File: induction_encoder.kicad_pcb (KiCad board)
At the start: 4 copper layers, 136 x 136 mm, 72 parts, among them J2 Conn_01x06, U1 MT9105ET, U10 IPS2200, U11 ADS1115IDGS, U12 ADS1115IDGS, U2 MT9105ET, U3 MT9105ET, U4 MT9105ET, U5 MT9105ET, U6 MT9105ET, U7 ADS1115IDGS, U8 MT9105ET, U9 MT9105ET

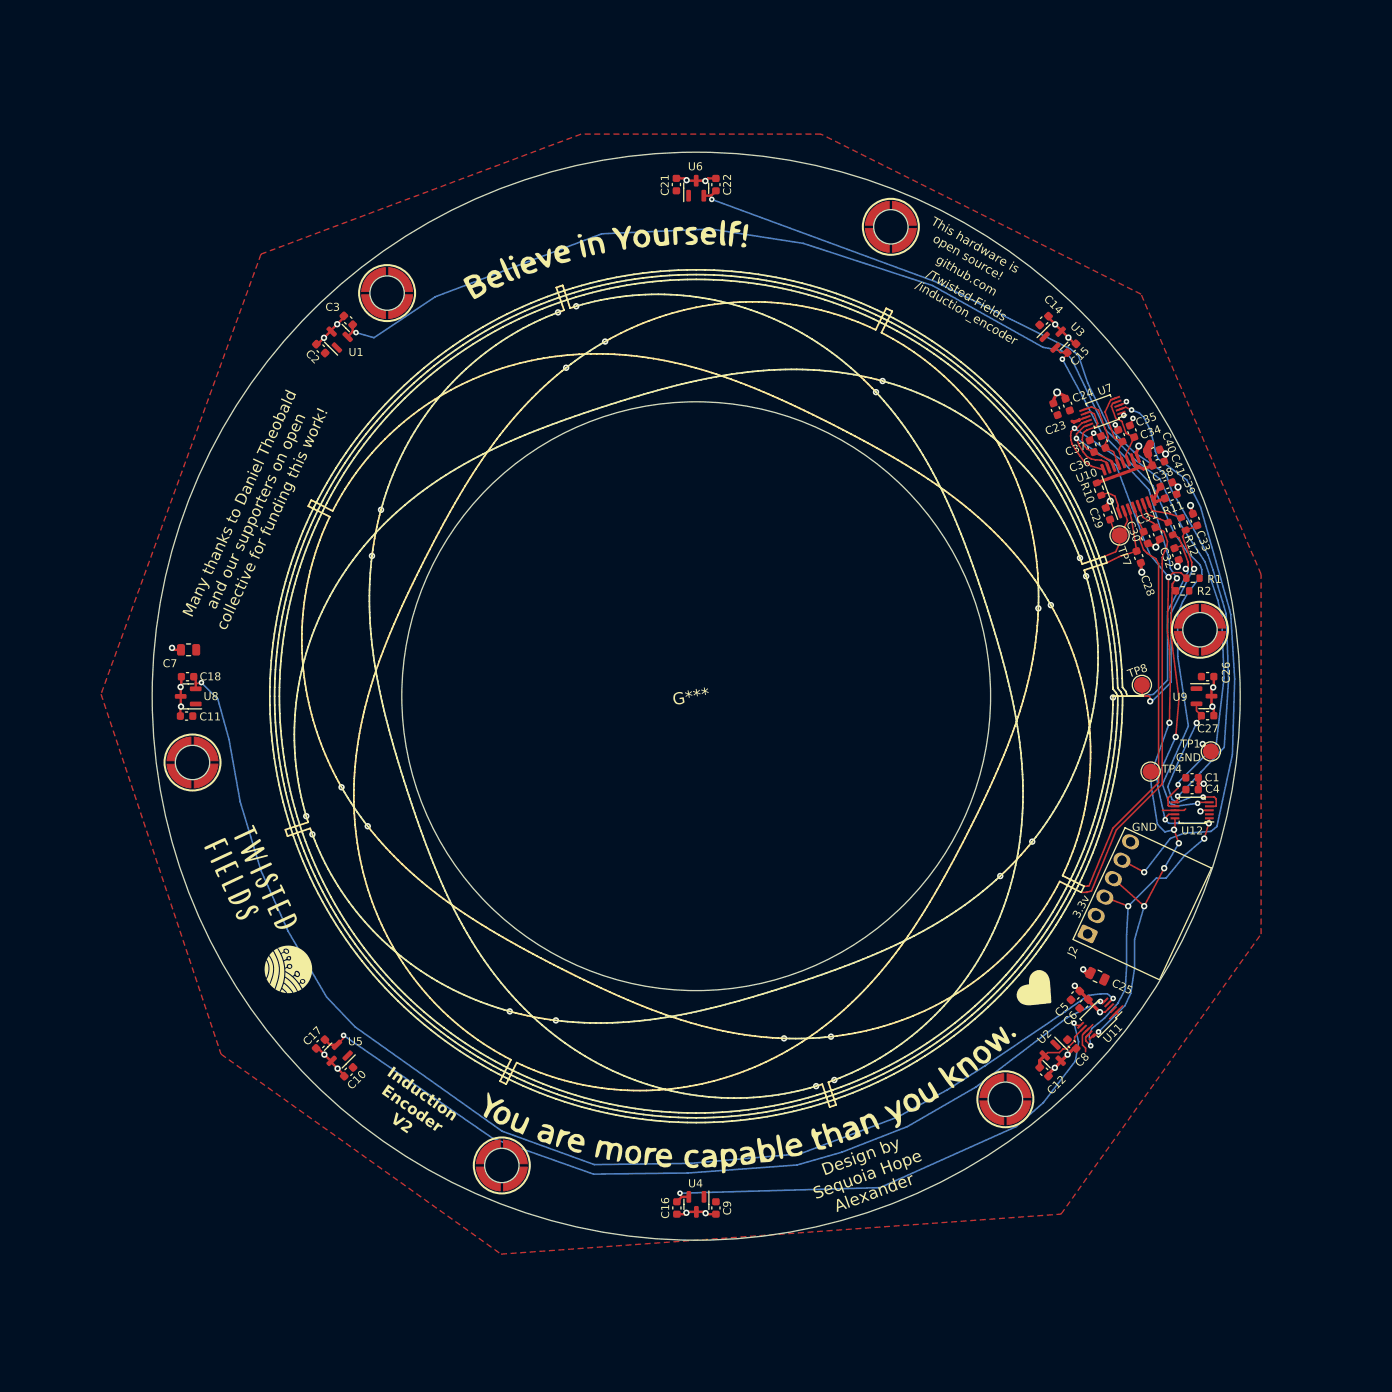
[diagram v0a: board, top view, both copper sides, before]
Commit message: changes for the 170mm design
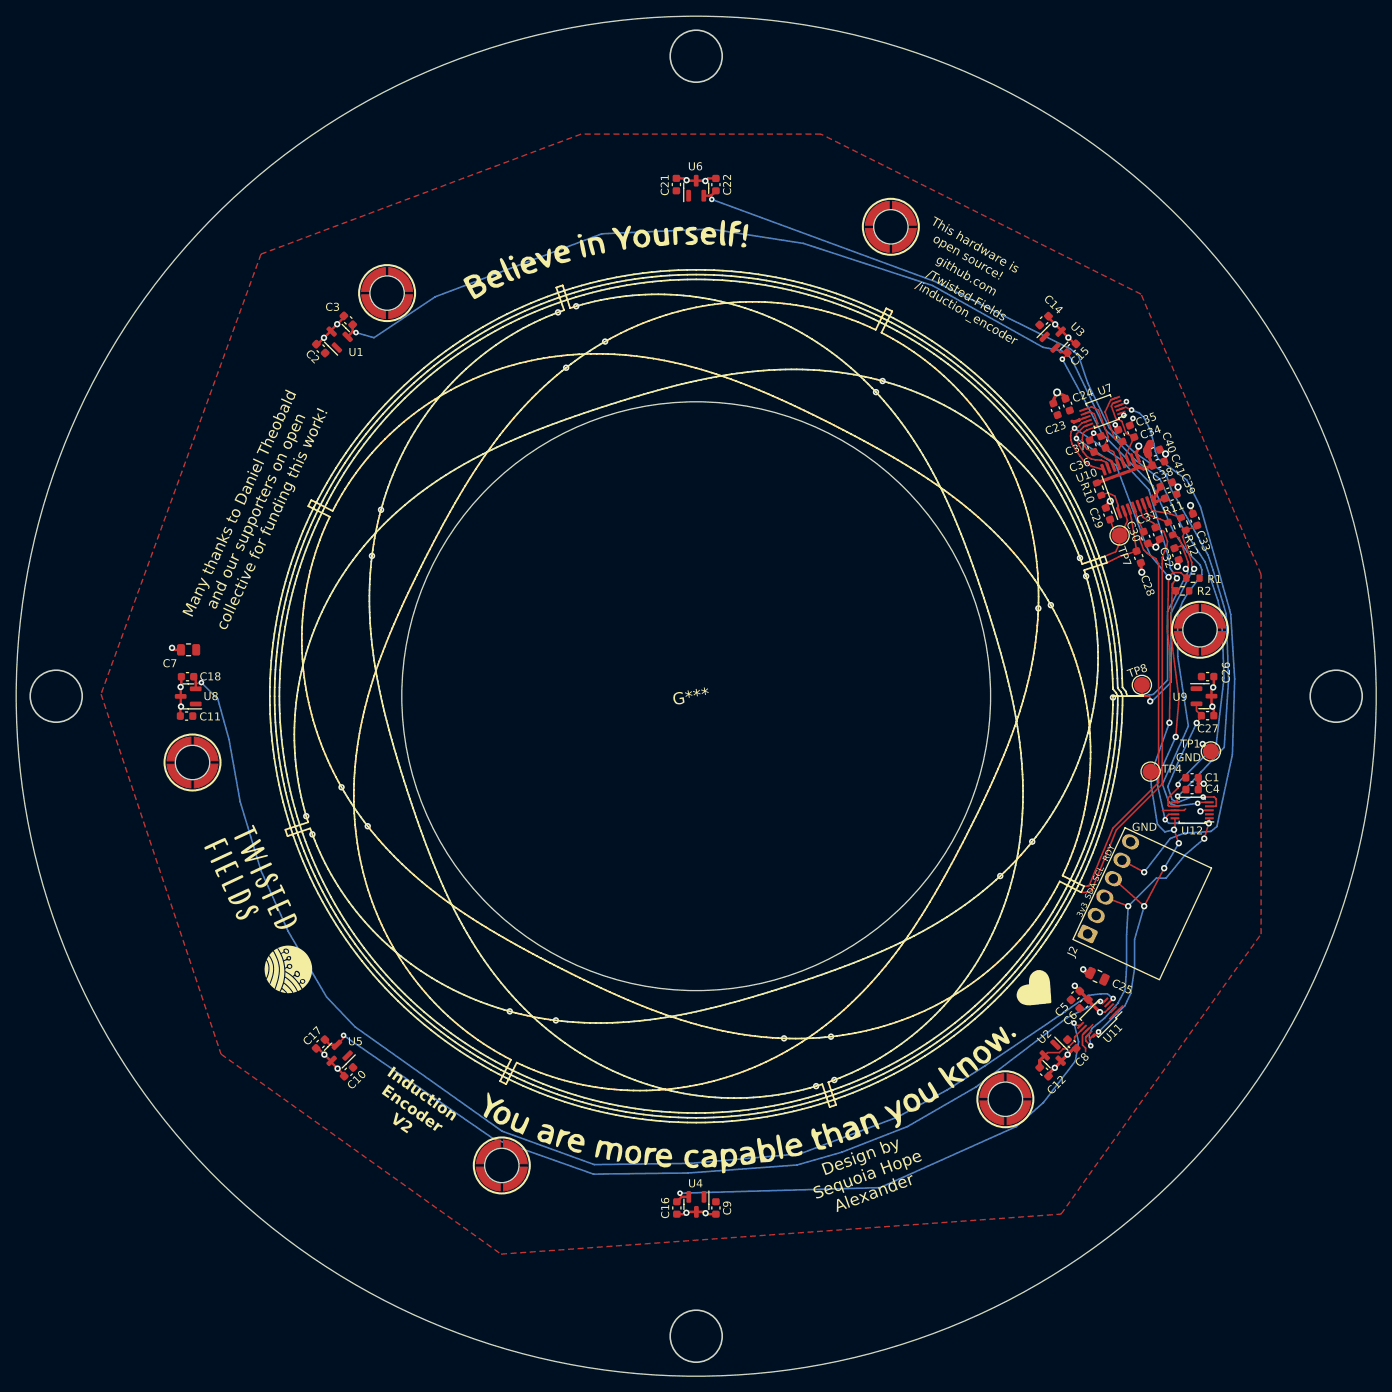
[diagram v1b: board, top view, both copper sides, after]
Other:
- board size 136 x 136 mm -> 170 x 170 mm
- board text added: "3v3"
- board text added: "RDY"
- board text added: "SCL"
- board text added: "SDA"
- board text removed: "3.3v"
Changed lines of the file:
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@@
 		(sheetname "Root")
 		(sheetfile "induction_encoder.kicad_sch")
-		(attr through_hole)
+		(attr through_hole dnp)
 		(fp_line
 			(start -1.4 -1)
@@
 	)
 	(gr_circle
+		(center 180 100)
+		(end 183.25 100)
+		(stroke
+			(width 0.2)
+			(type default)
+		)
+		(fill none)
+		(layer "Edge.Cuts")
+	)
+	(gr_circle
 		(center 100 100)
-		(end 168 100)
+		(end 185 100)
 		(stroke
 			(width 0.05)
@@
 	)
 	(gr_circle
+		(center 100 180)
+		(end 103.25 180)
+		(stroke
+			(width 0.2)
+			(type default)
+		)
+		(fill none)
+		(layer "Edge.Cuts")
+	)
+	(gr_circle
+		(center 20 100)
+		(end 23.25 100)
+		(stroke
+			(width 0.2)
+			(type default)
+		)
+		(fill none)
+		(layer "Edge.Cuts")
+	)
+	(gr_circle
+		(center 100 20)
+		(end 103.25 20)
+		(stroke
+			(width 0.2)
+			(type default)
+		)
+		(fill none)
+		(layer "Edge.Cuts")
+	)
+	(gr_circle
 		(center 100 100)
 		(end 100 136.8)
@@
 		(layer "Edge.Cuts")
 	)
+	(gr_text "RDY"
+		(at 151.5 120.75 65)
+		(layer "F.SilkS")
+		(effects
+			(font
+				(size 0.75 0.75)
+				(thickness 0.15)
+			)
+			(justify left bottom)
+		)
+	)
 	(gr_text "github.com"
 		(at 133.804938 47.434149 -30)
@@
 		)
 	)
+	(gr_text "SDA"
+		(at 149.25 125.5 65)
+		(layer "F.SilkS")
+		(effects
+			(font
+				(size 0.75 0.75)
+				(thickness 0.15)
+			)
+			(justify left bottom)
+		)
+	)
+	(gr_text "SCL"
+		(at 150.25 123.25 65)
+		(layer "F.SilkS")
+		(effects
+			(font
+				(size 0.75 0.75)
+				(thickness 0.15)
+			)
+			(justify left bottom)
+		)
+	)
 	(gr_text "Many thanks to Daniel Theobald\nand our supporters on open\ncollective for funding this work!"
 		(at 44.972085 76.853231 65)
@@
 		)
 	)
-	(gr_text "3.3v"
-		(at 147.943567 127.891336 62.5)
+	(gr_text "3v3"
+		(at 148.25 127.75 65)
 		(layer "F.SilkS")
 		(effects
 			(font
-				(size 1 1)
+				(size 0.75 0.75)
 				(thickness 0.15)
 			)
